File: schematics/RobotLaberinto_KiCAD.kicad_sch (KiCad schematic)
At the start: 9 parts, among them J1 ALIM_EDU_CIAA

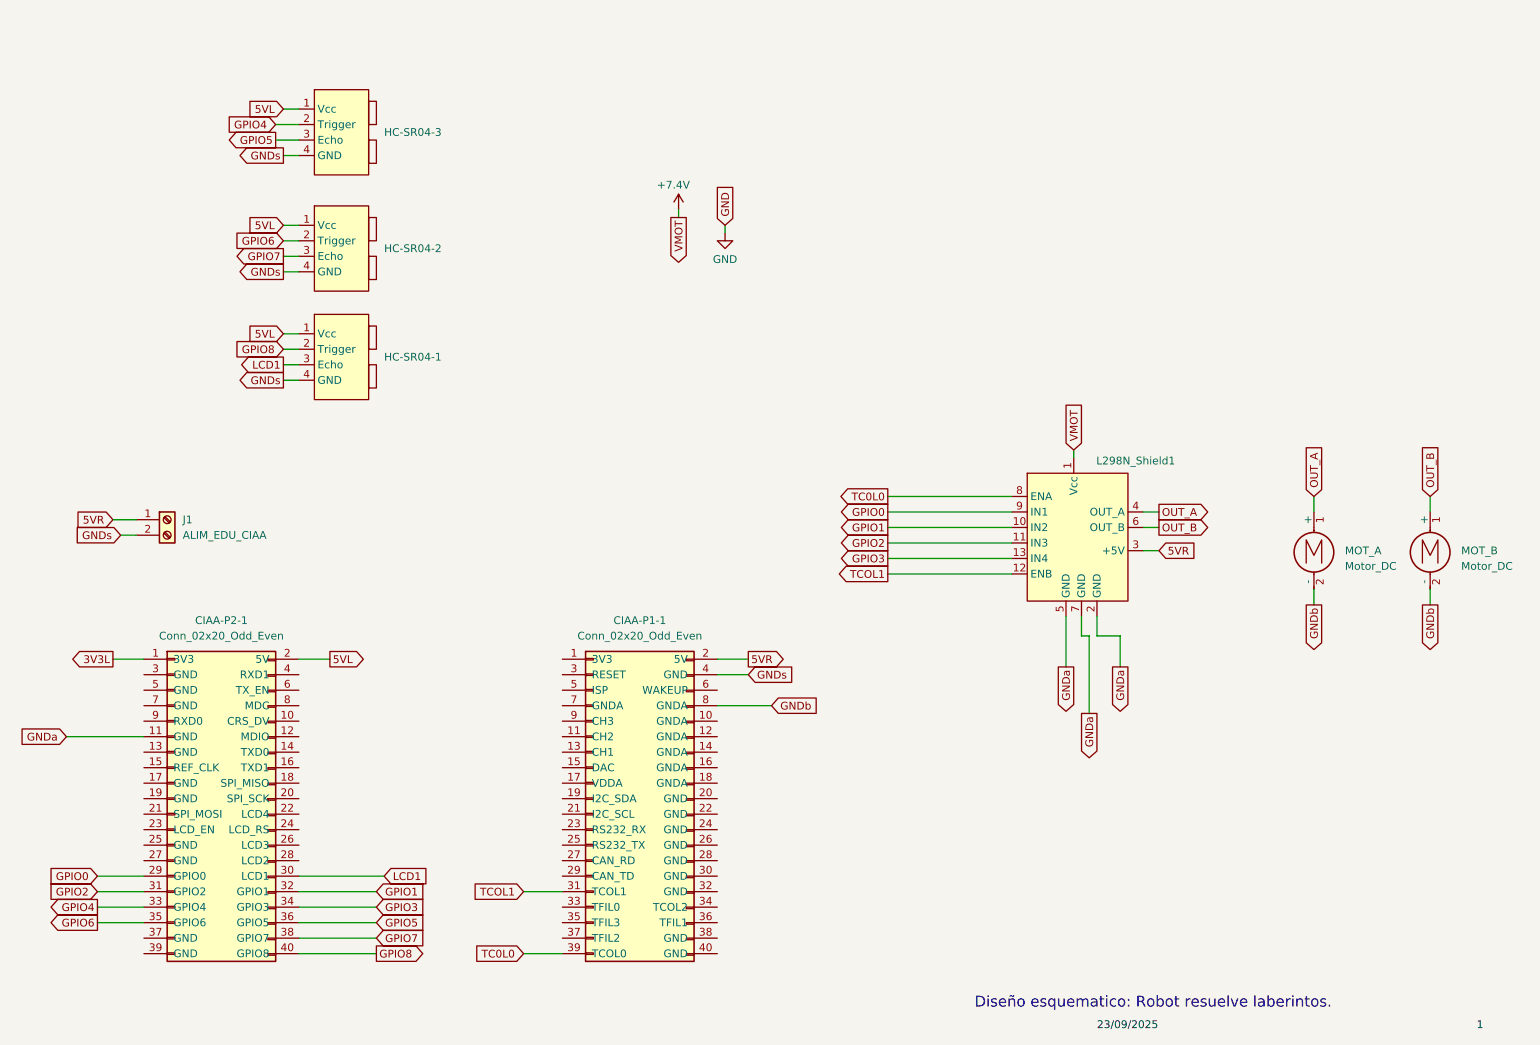
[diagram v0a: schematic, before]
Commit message: updt schematics
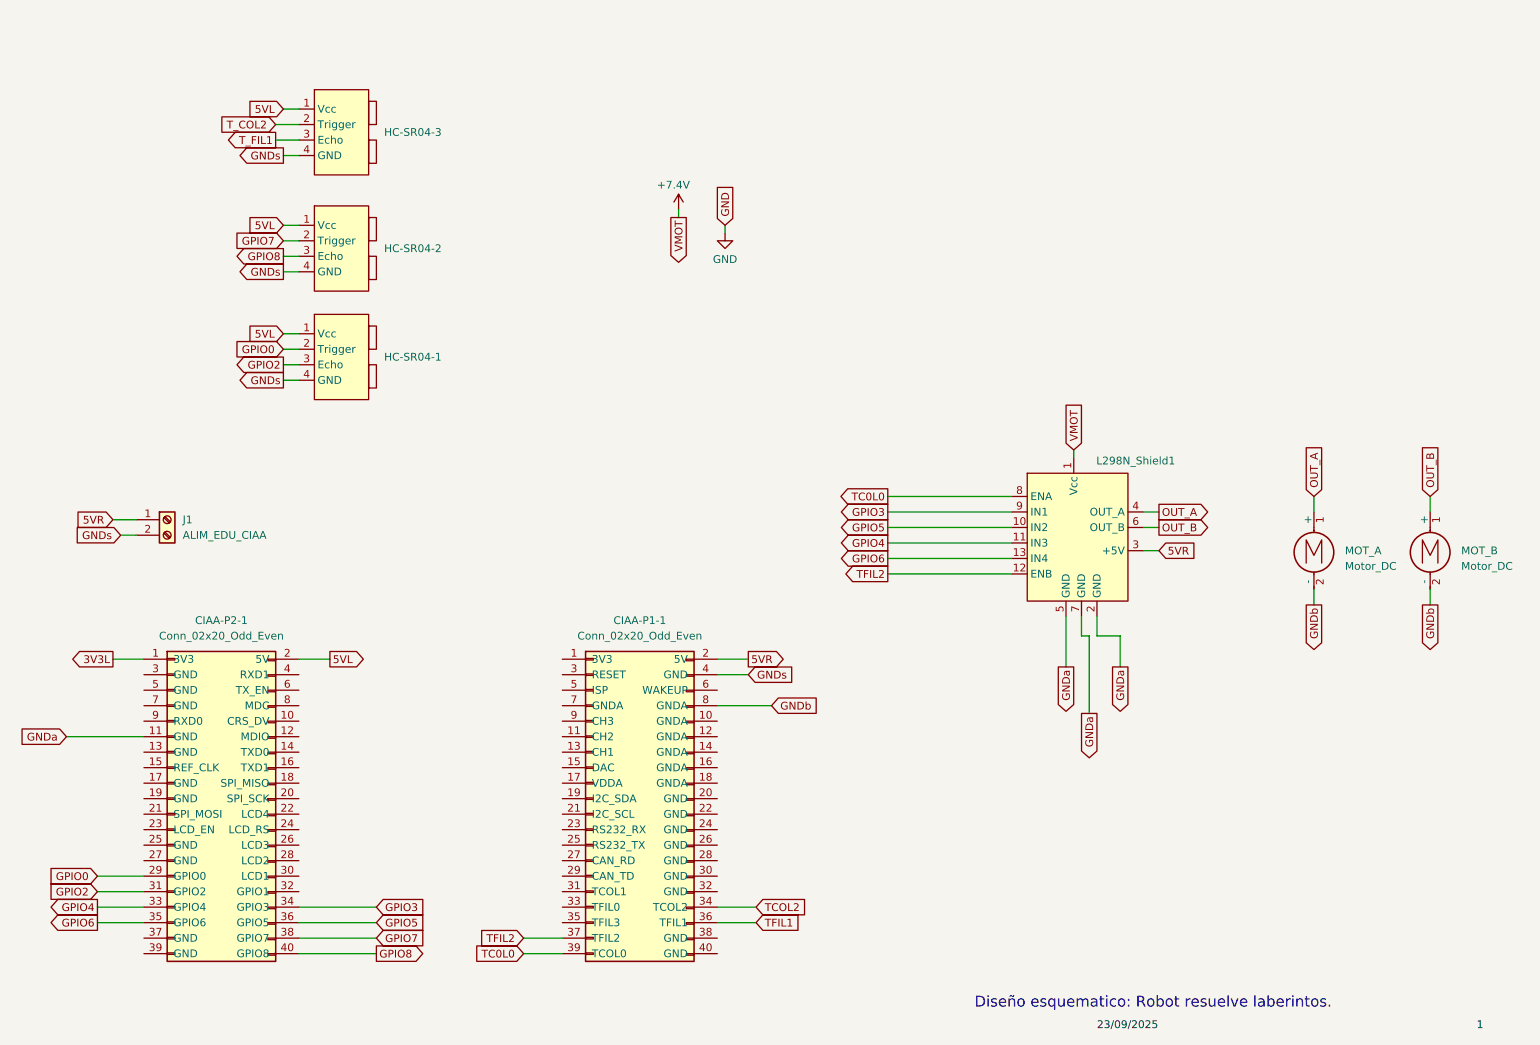
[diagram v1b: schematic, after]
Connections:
- net GPIO0: now also HC-SR04-1.2 (Trigger); no longer L298N_Shield1.9 (IN1)
- net GPIO2: now also HC-SR04-1.3 (Echo); no longer L298N_Shield1.11 (IN3)
- net GPIO3: now also L298N_Shield1.9 (IN1); no longer L298N_Shield1.13 (IN4)
- net GPIO4: now also L298N_Shield1.11 (IN3); no longer HC-SR04-3.2 (Trigger)
- net GPIO5: now also L298N_Shield1.10 (IN2); no longer HC-SR04-3.3 (Echo)
- net GPIO6: now also L298N_Shield1.13 (IN4); no longer HC-SR04-2.2 (Trigger)
- net GPIO7: now also HC-SR04-2.2 (Trigger); no longer HC-SR04-2.3 (Echo)
- net GPIO8: now also HC-SR04-2.3 (Echo); no longer HC-SR04-1.2 (Trigger)
- net TCOL2: now reaches CIAA-P1-1.34 (TCOL2)
- net TFIL1: now reaches CIAA-P1-1.36 (TFIL1)
- net TFIL2: now reaches CIAA-P1-1.37 (TFIL2)
- net TFIL2: now also L298N_Shield1.12 (ENB)
- net GPIO1: no longer names the net of CIAA-P2-1.32 (GPIO1)
- net GPIO1: no longer L298N_Shield1.10 (IN2)
- net LCD1: no longer names the net of CIAA-P2-1.30 (LCD1)
- net LCD1: no longer HC-SR04-1.3 (Echo)
- net TCOL1: no longer names the net of CIAA-P1-1.31 (TCOL1)
- net TCOL1: no longer L298N_Shield1.12 (ENB)
- new net T_COL2: HC-SR04-3.2 (Trigger)
- new net T_FIL1: HC-SR04-3.3 (Echo)

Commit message: schematic fixes
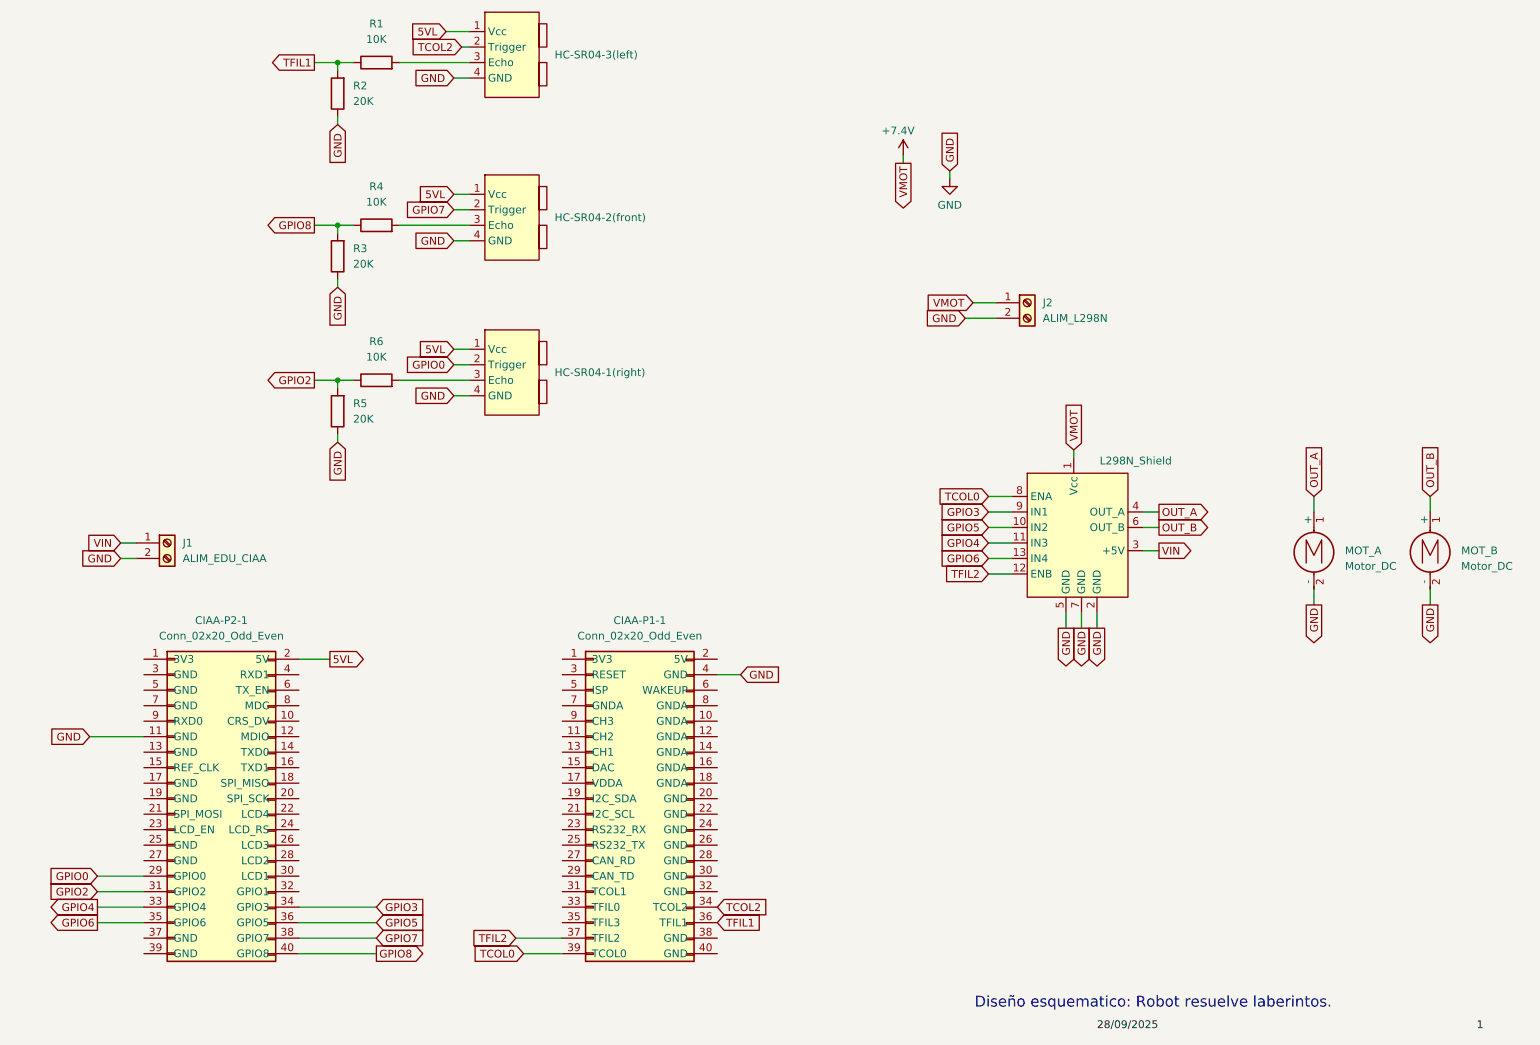
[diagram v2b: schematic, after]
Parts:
- added J2: ALIM_L298N, symbol Connector:Screw_Terminal_01x02
- added R1, R4, R6: 10K, symbol Device:R
- added R2, R3, R5: 20K, symbol Device:R
- renumbered HC-SR04-1 to HC-SR04-1(right), HC-SR04-2 to HC-SR04-2(front), HC-SR04-3 to HC-SR04-3(left), L298N_Shield1 to L298N_Shield
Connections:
- net GNDa is gone; now on net GND: CIAA-P2-1.11 (GND), L298N_Shield.2 (GND), L298N_Shield.5 (GND), L298N_Shield.7 (GND)
- net GNDs is gone; now on net GND: CIAA-P1-1.4 (GND), HC-SR04-1(right).4 (GND), HC-SR04-2(front).4 (GND), HC-SR04-3(left).4 (GND), J1.2 (Pin_2)
- net T_COL2 is gone; now on net TCOL2: HC-SR04-3(left).2 (Trigger)
- net +7.4V: now also J2.1 (Pin_1)
- net GND: now also MOT_A.2 (-), MOT_B.2 (-), J2.2 (Pin_2), R2.1, R3.1, R5.1
- net GPIO2: now also R5.2, R6.1; no longer HC-SR04-1(right).3 (Echo)
- net GPIO8: now also R3.2, R4.1; no longer HC-SR04-2(front).3 (Echo)
- net TFIL1: now also R1.1, R2.2
- net 3V3L: no longer names the net of CIAA-P2-1.1 (3V3)
- net 5VR renamed VIN
- net VIN: no longer CIAA-P1-1.2 (5V)
- removed net GNDb: CIAA-P1-1.8 (GNDA), MOT_A.2 (-), MOT_B.2 (-)
- net TC0L0 renamed TCOL0
- net T_FIL1: no longer names the net of HC-SR04-3(left).3 (Echo)
- net T_FIL1: now also R1.2
- new net: HC-SR04-2(front).3 (Echo), R4.2
- new net: HC-SR04-1(right).3 (Echo), R6.2
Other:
- moved on the sheet: HC-SR04-1(right), HC-SR04-2(front), HC-SR04-3(left), J1
